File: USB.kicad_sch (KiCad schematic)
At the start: 8 parts, among them J23 USB_B_Micro, U19 CP2102N-A02-GQFN24

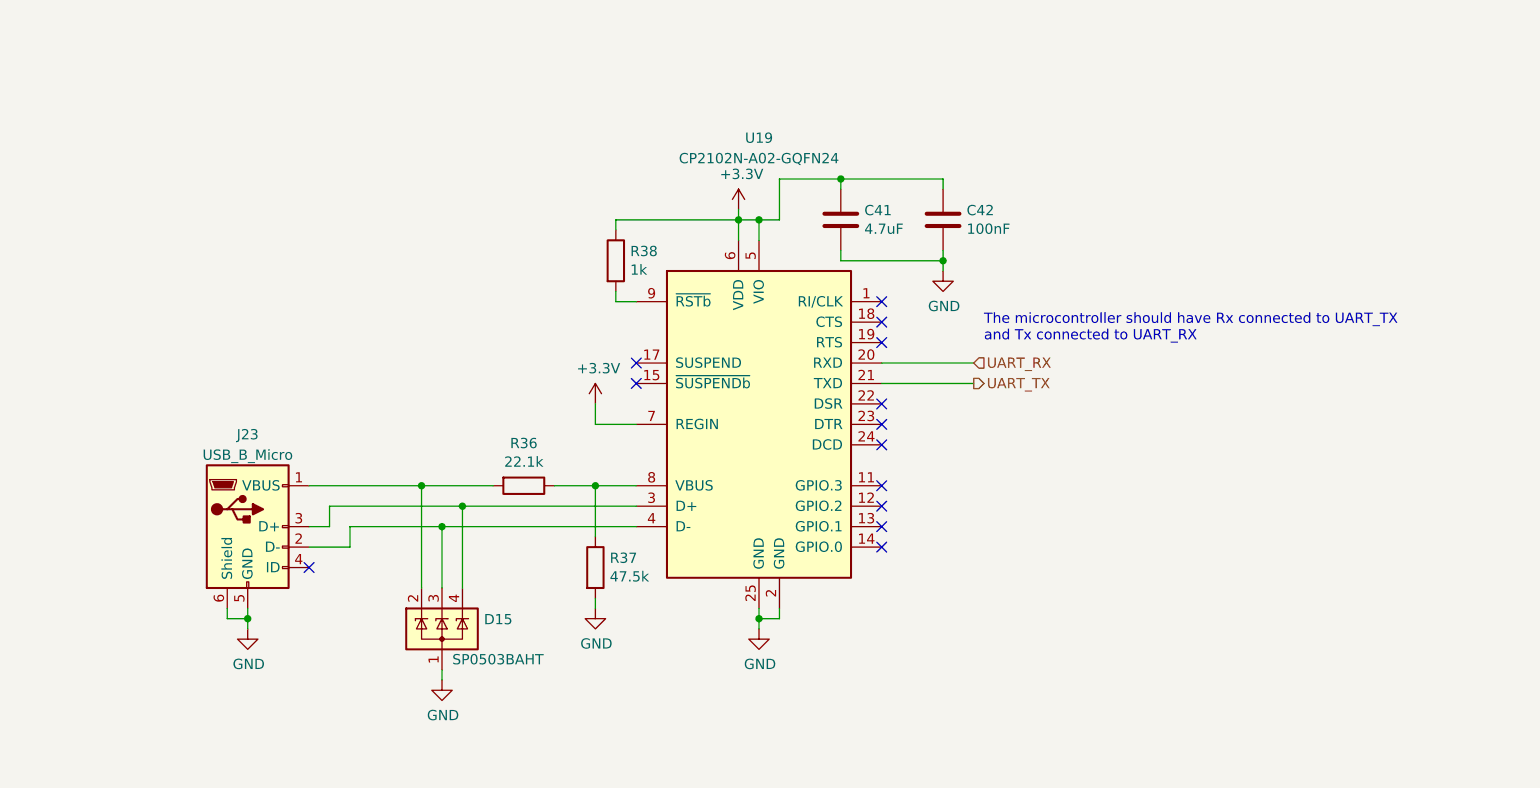
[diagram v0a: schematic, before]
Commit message: v1.2 initial changes
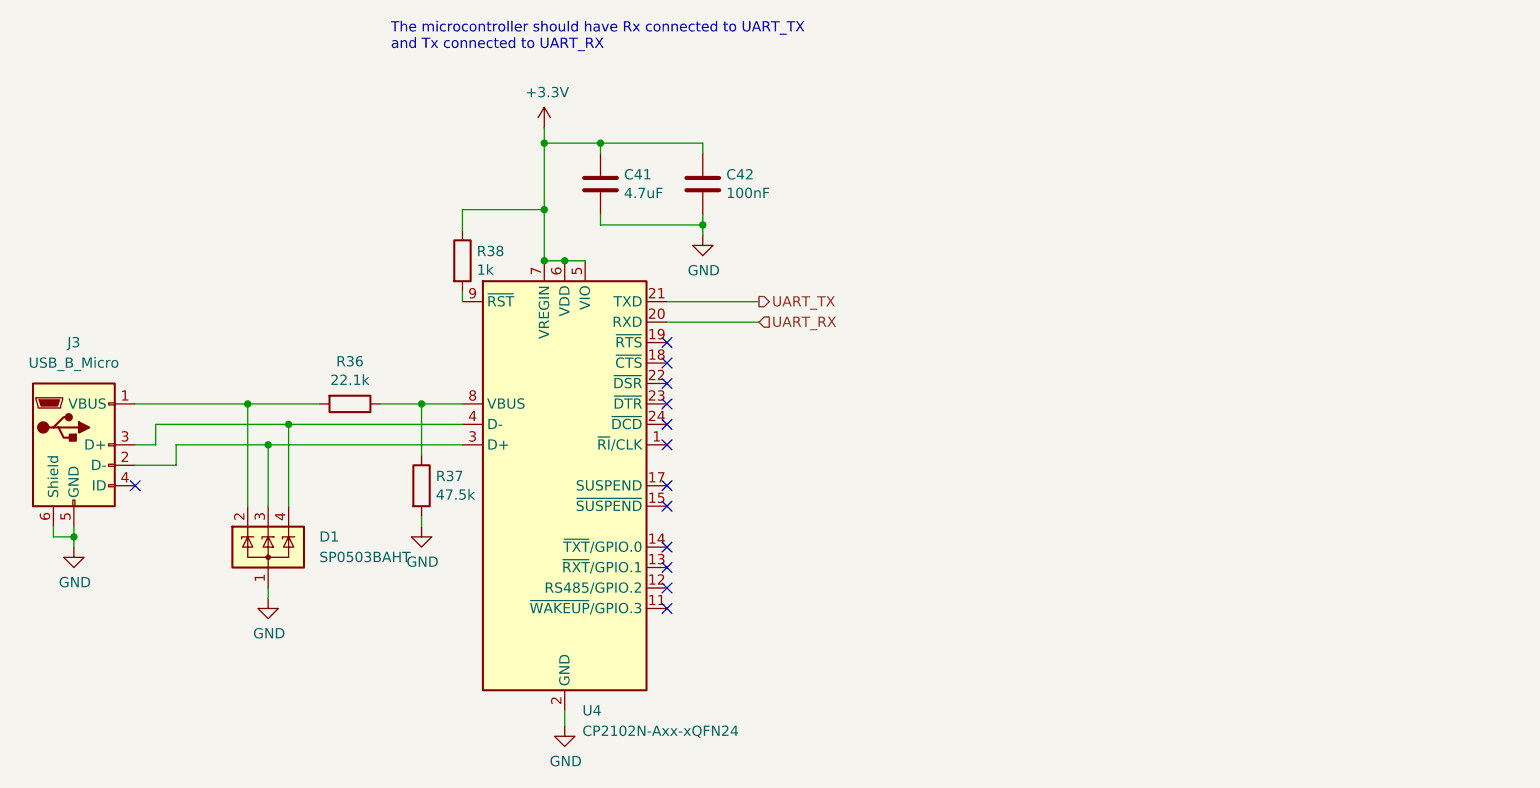
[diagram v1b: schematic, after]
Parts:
- removed D15: SP0503BAHT, Package_TO_SOT_SMD:SOT-143, symbol Dash2-rescue:SP0503BAHT-Power_Protection
- removed J23: USB_B_Micro, Connector_USB:USB_Micro-B_Molex-105017-0001, symbol Dashboard-rescue:USB_B_Micro-Connector
- removed U19: CP2102N-A02-GQFN24, Package_DFN_QFN:QFN-24-1EP_4x4mm_P0.5mm_EP2.6x2.6mm, symbol Interface_USB:CP2102N-A01-GQFN24
- added D1: SP0503BAHT, Package_TO_SOT_SMD:SOT-143, symbol Power_Protection:SP0503BAHT
- added J3: USB_B_Micro, Connector_USB:USB_Micro-B_Molex-105017-0001, symbol Connector:USB_B_Micro
- added U4: CP2102N-Axx-xQFN24, Package_DFN_QFN:QFN-24-1EP_4x4mm_P0.5mm_EP2.6x2.6mm, symbol Interface_USB:CP2102N-Axx-xQFN24
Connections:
- net +3.3V: now also U4.5 (VIO), U4.6 (VDD), U4.7 (VREGIN)
- net GND: now also D1.1 (A), J3.5 (GND), J3.6 (Shield), U4.2 (GND), U4.25 (GND)
- net UART_RX: now also U4.20 (RXD)
- net UART_TX: now also U4.21 (TXD)
- net at R36.1, R37.1: now also U4.8 (VBUS)
- net at R36.2: now also D1.2 (K), J3.1 (VBUS)
- net at R38.2: now also U4.9 (~{RST})
- new net: D1.3 (K), J3.2 (D-), U4.3 (D+)
- new net: D1.4 (K), J3.3 (D+), U4.4 (D-)
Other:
- moved on the sheet: C41, C42, R36, R37, R38
